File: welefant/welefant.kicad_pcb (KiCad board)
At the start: 2 copper layers, 80 x 90 mm, 72 parts, among them J1 Conn_02x11_Odd_Even, J2 Conn_02x11_Odd_Even, Q1 AO3400A, Q2 AO3401A, Q3 AO3401A, Q4 AO3400A, SW1 TS-1187A-B-A-B, SW2 TS-1187A-B-A-B, U1 ESP32-S3-WROOM-1-N8, U2 welefant, U3 XB8089D, U4 TP4056, U5 HE9073A33M5R, U6 MT3608L, U7 SK6812MINI-E_C5149201, U8 SK6812MINI-E_C5149201

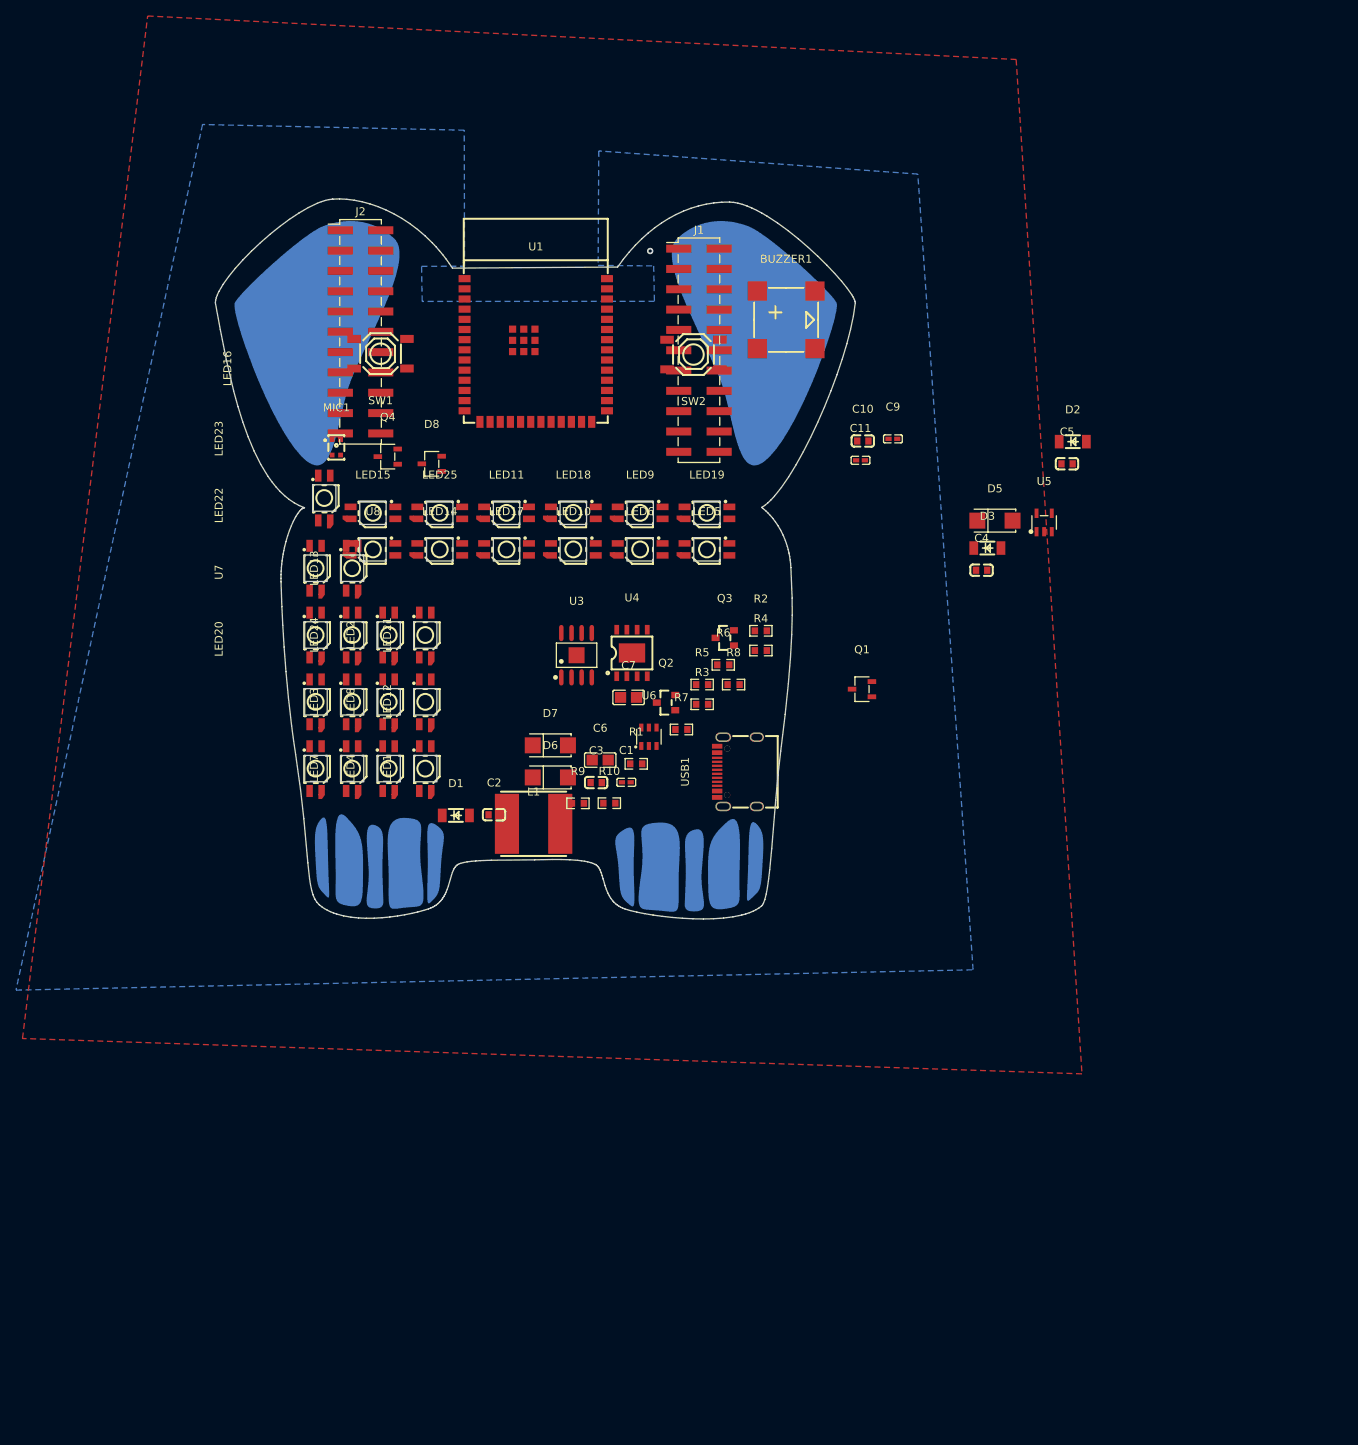
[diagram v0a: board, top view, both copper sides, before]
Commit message: blubb
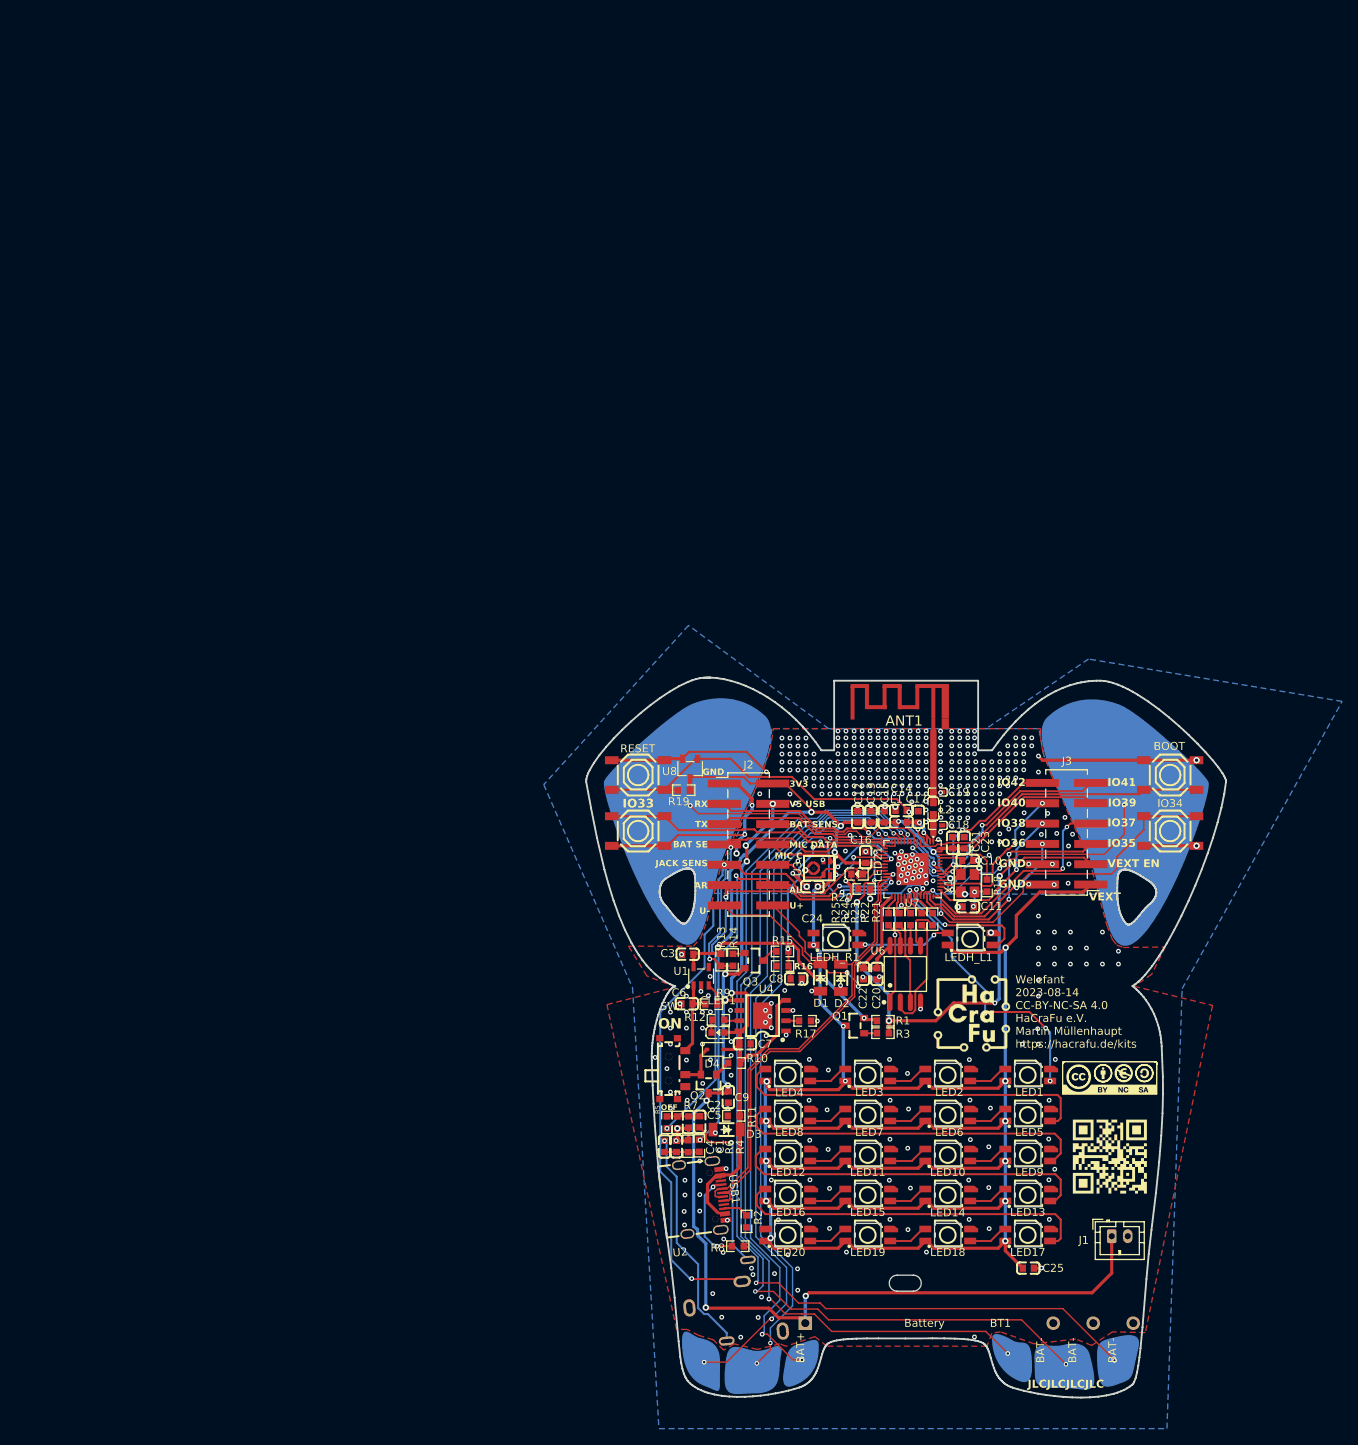
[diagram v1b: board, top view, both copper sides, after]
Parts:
- removed BUZZER1: MLT-8530, easyeda2kicad:BUZ-SMD_4P-L8.5-W8.5-P8.50-TL
- removed D5, D6, D7: SS34, easyeda2kicad:SMA_L4.3-W2.6-LS5.2-RD
- removed D8: BAV99,215, easyeda2kicad:SOT-23-3_L2.9-W1.6-P1.90-LS2.8-BR
- removed LED22, LED23, LED24, LED25: SK6812MINI-E, hacrafu:SK6812MINI-E-handsolder
- removed MIC1: ZTS6117, easyeda2kicad:MIC-SMD_4P-L2.8-W1.9-P1.84-TL_ZTS6117
- removed Q4: AO3400A, easyeda2kicad:SOT-23-3_L2.9-W1.6-P1.90-LS2.8-BR
- added ANT1: ANTENNA, hacrafu:antenna, F.Cu at (71.3, 36.8)
- added BT1: Battery, hacrafu:LiPo_Recycled_welefant, F.Cu at (59.4, 114.0)
- added C12: 10u, easyeda2kicad:C0603, F.Cu at (66.0, 50.7)
- added C13: 1u, easyeda2kicad:C0603, F.Cu at (67.6, 50.7)
- added C14: 1u, easyeda2kicad:C0603, F.Cu at (71.4, 49.9)
- added C15: 100n, easyeda2kicad:C0603, F.Cu at (69.3, 50.7)
- added C16: 100n, easyeda2kicad:C0603, F.Cu at (67.0, 55.8)
- added C17: 100n, easyeda2kicad:C0603, F.Cu at (73.5, 50.7)
- added C18: 4p7, easyeda2kicad:C0402, F.Cu at (76.0, 51.8)
- added C19: 3p3, easyeda2kicad:C0402, F.Cu at (76.0, 47.6)
- added C20: 100n, easyeda2kicad:C0603, F.Cu at (68.3, 70.3)
- added C21: 100n, easyeda2kicad:C0603, F.Cu at (77.8, 54.0)
- added C22: 1u, easyeda2kicad:C0603, F.Cu at (66.7, 70.3)
- added C23: 100n, easyeda2kicad:C0603, F.Cu at (79.2, 54.0)
- added C24: 100n, easyeda2kicad:C0603, F.Cu at (60.3, 59.5)
- added C25: 1u, easyeda2kicad:C0603, F.Cu at (87.3, 107.1)
- added C8: 10u, easyeda2kicad:C0603, F.Cu at (58.2, 71.0)
- added CLED1: yellow, easyeda2kicad:LED0603-RD-YELLOW, F.Cu at (48.5, 77.7)
- added D4: 1N5819WS, Diode_SMD:D_SOD-323, F.Cu at (48.1, 79.8)
- added J3: Conn_02x6_Odd_Even, hacrafu:PinHeader_2x06_P2.54mm_Vertical_SMD_handsolder, F.Cu at (92.0, 50.3)
- added L2: 2n2, easyeda2kicad:L0603, F.Cu at (75.4, 49.7)
- added LEDH_L1: SK6812MINI-E, hacrafu:SK6812MINI-E-handsolder, F.Cu at (80.0, 66.0)
- added LEDH_R1: SK6812MINI-E, hacrafu:SK6812MINI-E-handsolder, F.Cu at (63.2, 66.0)
- added R11: 10K, easyeda2kicad:R0603, F.Cu at (50.5, 88.1)
- added R12: 330, easyeda2kicad:R0603, F.Cu at (48.5, 76.1)
- added R13: 10K, easyeda2kicad:R0603, F.Cu at (48.9, 68.6)
- added R14: 1K, easyeda2kicad:R0603, F.Cu at (50.4, 68.6)
- added R15: 390K, easyeda2kicad:R0603, F.Cu at (56.5, 67.5)
- added R16: 100K, easyeda2kicad:R0603, F.Cu at (56.5, 69.4)
- added R17: 3K3, easyeda2kicad:R0603_NEW, F.Cu at (59.4, 76.2)
- added R18: 0, easyeda2kicad:R0603, F.Cu at (82.1, 59.3)
- added R19: 10K, easyeda2kicad:R0603, F.Cu at (44.2, 47.4)
- added R20: 330, easyeda2kicad:R0603, F.Cu at (66.8, 59.8)
- added R21: 0, easyeda2kicad:R0603, F.Cu at (75.3, 63.5)
- added R22: 0, easyeda2kicad:R0603, F.Cu at (74.0, 63.5)
- added R23: 0, easyeda2kicad:R0603, F.Cu at (72.5, 63.5)
- added R24: 0, easyeda2kicad:R0603, F.Cu at (71.2, 63.5)
- added R25: 0, easyeda2kicad:R0603, F.Cu at (69.8, 63.5)
- added SW3: BOOT, easyeda2kicad:SW-SMD_4P-L5.1-W5.1-P3.70-LS6.5-TL-2, F.Cu at (105.0, 45.5)
- added SW4: GPIO33, easyeda2kicad:SW-SMD_4P-L5.1-W5.1-P3.70-LS6.5-TL-2, F.Cu at (38.5, 52.5)
- added SW5: IO34, easyeda2kicad:SW-SMD_4P-L5.1-W5.1-P3.70-LS6.5-TL-2, F.Cu at (105.0, 52.5)
- added X1: 40 MHz, easyeda2kicad:OSC-SMD_4P-L3.2-W2.5-BL_SIT8008BI, F.Cu at (79.7, 59.0)
- C1: value 0.1u -> 33n; footprint easyeda2kicad:C0402_NEW -> easyeda2kicad:C0603
- C10: value 10u -> 15p
- C11: value 0.1u -> 15p; footprint easyeda2kicad:C0402_NEW -> easyeda2kicad:C0603
- C2: value 10u -> 33n
- C6: value 22u -> 1u; footprint easyeda2kicad:C0805 -> easyeda2kicad:C0603
- C7: value 22u -> 10u; footprint easyeda2kicad:C0805 -> easyeda2kicad:C0603
- C9: value 0.1u -> 10u; footprint easyeda2kicad:C0402_NEW -> easyeda2kicad:C0603
- D1: value 5V6 -> 3V3
- D3: value 3V3 -> 5V6
- J1: value Conn_02x11_Odd_Even -> Conn_01x02; footprint Connector_PinHeader_2.54mm:PinHeader_2x11_P2.54mm_Vertical_SMD -> Connector_JST:JST_PH_B2B-PH-K_1x02_P2.00mm_Vertical
- J2: value Conn_02x11_Odd_Even -> Conn_02x7_Odd_Even; footprint Connector_PinHeader_2.54mm:PinHeader_2x11_P2.54mm_Vertical_SMD -> hacrafu:PinHeader_2x07_P2.54mm_Vertical_SMD_handsolder
- L1: value 10u -> 2n2; footprint easyeda2kicad:IND-SMD_L8.0-W8.0 -> easyeda2kicad:L0603
- LED21: value SK6812MINI-E -> blue; footprint hacrafu:SK6812MINI-E-handsolder -> easyeda2kicad:LED0603-FD_BLUE
- Q1: value AO3400A -> AO3401A; footprint easyeda2kicad:SOT-23-3_L2.9-W1.6-P1.90-LS2.8-BR -> easyeda2kicad:SOT-23_L2.9-W1.3-P1.90-LS2.4-BR
- R1: value 5.1K -> 10K
- R10: value 10K -> 1K
- R2: value 1K -> 5.1K
- R3: value 5.1K -> 1K
- R4, R5: value 2.4K -> 270
- R6: value 10K -> 150
- R7: value 110K -> 150
- R8: value 110K -> 5.1K
- R9: value 15K -> 100K
- SW1: value TS-1187A-B-A-B -> ON-OFF; footprint easyeda2kicad:SW-SMD_4P-L5.1-W5.1-P3.70-LS6.5-TL-2 -> easyeda2kicad:SW-TH_K3-1296S-E1
- SW2: value TS-1187A-B-A-B -> RESET
- U1: value ESP32-S3-WROOM-1-N8 -> RT9080-33GJ5; footprint easyeda2kicad:WIFIM-SMD_ESP32-S3-WROOM-1-N8 -> easyeda2kicad:TSOT-23-5_L2.9-W1.6-P0.95-LS2.8-BL
- U2: value welefant -> Audio Jack PJ-324; footprint hacrafu:welefant -> easyeda2kicad:AUDIO-TH_PJ-32400
- U3: value XB8089D -> SD18OB261-060; footprint easyeda2kicad:SOIC-8_L5.0-W4.0-P1.27-LS6.0-BL-EP2.0 -> hacrafu:MIC-SMD_SD18OB261-060
- U5: value HE9073A33M5R -> welefant; footprint easyeda2kicad:SOT-23-5_L3.0-W1.7-P0.95-LS2.8-BL -> hacrafu:welefant; moved to B.Cu
- U6: value MT3608L -> 128MBit Flash; footprint easyeda2kicad:SOT-23-6_L2.9-W1.7-P0.95-LS2.8-BL -> easyeda2kicad:SOIC-8_L5.3-W5.3-P1.27-LS8.0-BL
- U7: value SK6812MINI-E_C5149201 -> ESP32-S3; footprint hacrafu:SK6812MINI-E-handsolder -> easyeda2kicad:QFN-56_L7.0-W7.0-P0.40-TL-EP4.0
- U8: value SK6812MINI-E_C5149201 -> Reset 2.8V; footprint hacrafu:SK6812MINI-E-handsolder -> easyeda2kicad:SOT-23-3_L2.9-W1.6-P1.90-LS2.8-BR
- moved J1 122.2 mm to (97.7, 103.2)
- moved LED13 115.2 mm to (87.2, 98.0), turned to 180 degrees
- moved LED17 107.7 mm to (87.2, 103.0), turned to 180 degrees
- moved LED15 105.3 mm to (67.2, 98.0), turned to 180 degrees
- moved LED16 104.6 mm to (57.2, 98.0), turned to 180 degrees
- moved LED14 102.7 mm to (77.2, 98.0), turned to 180 degrees
- moved LED18 101.7 mm to (77.2, 103.0), turned to 180 degrees
- moved SW1 96.5 mm to (42.8, 82.2), turned to 0 degrees
- moved U2 96.0 mm to (50.5, 111.2), turned to 6 degrees
- moved C5 94.2 mm to (46.2, 88.8), turned to -90 degrees
- moved LED9 93.8 mm to (87.2, 93.0), turned to 180 degrees
- moved LED19 92.5 mm to (67.2, 103.0), turned to 180 degrees
- moved LED11 92.1 mm to (67.2, 93.0), turned to 180 degrees
- moved LED10 89.0 mm to (77.2, 93.0), turned to 180 degrees
- moved LED2 88.9 mm to (77.2, 83.0), turned to 180 degrees
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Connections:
- C1 pad 1: Net-(C1-Pad1) -> GND
- C10 pad 1: Net-(BUZZER1-Pad1) -> /XTAL_N
- C10 pad 2: /GND -> GND
- C11 pad 1: Net-(R14-Pad2) -> GND
- C2 pad 1: /Power/VBAT -> GND
- C2 pad 2: /GND -> Net-(C2-Pad2)
- C3 pad 1: /Power/VUSB -> GND
- C3 pad 2: /GND -> /V33
- C4 pad 1: Net-(Q2-Pad2) -> Net-(C1-Pad2)
- C4 pad 2: /GND -> Net-(C4-Pad2)
- C5 pad 1: /GND -> Net-(C2-Pad2)
- C5 pad 2: /Power/V33 -> Net-(C5-Pad2)
- C6 pad 1: /Power/V5 -> GND
- C6 pad 2: /GND -> /VBUS
- C7 pad 1: Net-(C7-Pad1) -> /V5
- C7 pad 2: /GND -> GND
- C9 pad 1: /VEXT -> GND
- C9 pad 2: /GND -> /VBAT
- D1 pad 1: /Power/VUSB -> /USB_DP
- D1 pad 2: /GND -> GND
- D2 pad 1: /Power/USB_DP -> /USB_DN
- D2 pad 2: /GND -> GND
- D3 pad 1: /Power/USB_DN -> /V5
- D3 pad 2: /GND -> GND
- J1 pad 1: unconnected-(J1-Pad1) -> /VBAT
- J1 pad 2: unconnected-(J1-Pad2) -> GND
- J2 pad 1: unconnected-(J2-Pad1) -> GND
- J2 pad 10: unconnected-(J2-Pad10) -> /MIC_CLK
- J2 pad 11: unconnected-(J2-Pad11) -> /AUDIO_PWM_R
- J2 pad 12: unconnected-(J2-Pad12) -> /AUDIO_PWM_L
- J2 pad 13: unconnected-(J2-Pad13) -> /USB_DP
- J2 pad 14: unconnected-(J2-Pad14) -> /USB_DN
- J2 pad 2: unconnected-(J2-Pad2) -> /V33
- J2 pad 3: unconnected-(J2-Pad3) -> /RX
- J2 pad 4: unconnected-(J2-Pad4) -> /V5
- J2 pad 5: unconnected-(J2-Pad5) -> /TX
- J2 pad 6: unconnected-(J2-Pad6) -> /BAT_SENS
- J2 pad 7: unconnected-(J2-Pad7) -> /BAT_SENS_EN
- J2 pad 8: unconnected-(J2-Pad8) -> /MIC_DATA
- J2 pad 9: unconnected-(J2-Pad9) -> /JACK_SENS
- L1 pad 1: Net-(D7-Pad2) -> /V33
- L1 pad 2: Net-(C7-Pad1) -> Net-(C17-Pad2)
- LED1 pad 1: /LEDs/VUSB -> /VEXT
- LED1 pad 2: unconnected-(LED1-Pad2) -> Net-(LED1-DOUT)
- LED1 pad 3: /LEDs/GND -> GND
- LED1 pad 4: Net-(LED1-Pad4) -> /LED_MATRIX
- LED10 pad 1: /LEDs/VUSB -> /VEXT
- LED10 pad 2: Net-(LED10-Pad2) -> Net-(LED10-DOUT)
- LED10 pad 3: /LEDs/GND -> GND
- LED10 pad 4: unconnected-(LED10-Pad4) -> Net-(LED10-DIN)
- LED11 pad 1: /LEDs/VUSB -> /VEXT
- LED11 pad 2: unconnected-(LED11-Pad2) -> Net-(LED11-DOUT)
- LED11 pad 3: /LEDs/GND -> GND
- LED11 pad 4: Net-(LED11-Pad4) -> Net-(LED10-DOUT)
- LED12 pad 1: /LEDs/VUSB -> /VEXT
- LED12 pad 2: Net-(LED11-Pad4) -> /D3_LED
- LED12 pad 3: /LEDs/GND -> GND
- LED12 pad 4: Net-(LED12-Pad4) -> Net-(LED11-DOUT)
- LED13 pad 1: /LEDs/VUSB -> /VEXT
- LED13 pad 2: Net-(LED12-Pad4) -> Net-(LED13-DOUT)
- LED13 pad 3: /LEDs/GND -> GND
- LED13 pad 4: Net-(LED13-Pad4) -> /D3_LED
- LED14 pad 1: /LEDs/VUSB -> /VEXT
- LED14 pad 2: Net-(LED13-Pad4) -> Net-(LED14-DOUT)
- LED14 pad 3: /LEDs/GND -> GND
- LED14 pad 4: Net-(LED14-Pad4) -> Net-(LED13-DOUT)
- LED15 pad 1: /LEDs/VUSB -> /VEXT
- LED15 pad 2: Net-(LED14-Pad4) -> Net-(LED15-DOUT)
- LED15 pad 3: /LEDs/GND -> GND
- LED15 pad 4: unconnected-(LED15-Pad4) -> Net-(LED14-DOUT)
- LED16 pad 1: /LEDs/VUSB -> /VEXT
- LED16 pad 2: unconnected-(LED16-Pad2) -> /D4_LED
- LED16 pad 3: /LEDs/GND -> GND
- LED16 pad 4: Net-(LED16-Pad4) -> Net-(LED15-DOUT)
- LED17 pad 1: /LEDs/VUSB -> /VEXT
- LED17 pad 2: Net-(LED16-Pad4) -> Net-(LED17-DOUT)
- LED17 pad 3: /LEDs/GND -> GND
- LED17 pad 4: Net-(LED17-Pad4) -> /D4_LED
- LED18 pad 1: /LEDs/VUSB -> /VEXT
- LED18 pad 2: Net-(LED17-Pad4) -> Net-(LED18-DOUT)
- LED18 pad 3: /LEDs/GND -> GND
- LED18 pad 4: Net-(LED18-Pad4) -> Net-(LED17-DOUT)
- LED19 pad 1: /LEDs/VUSB -> /VEXT
- LED19 pad 2: Net-(LED18-Pad4) -> Net-(LED19-DOUT)
- LED19 pad 3: /LEDs/GND -> GND
- LED19 pad 4: Net-(LED19-Pad4) -> Net-(LED18-DOUT)
- LED2 pad 1: /LEDs/VUSB -> /VEXT
- LED2 pad 2: Net-(LED1-Pad4) -> Net-(LED2-DOUT)
- LED2 pad 3: /LEDs/GND -> GND
- LED2 pad 4: Net-(LED2-Pad4) -> Net-(LED1-DOUT)
- LED20 pad 1: /LEDs/VUSB -> /VEXT
- LED20 pad 2: Net-(LED19-Pad4) -> unconnected-(LED20-DOUT-Pad2)
- LED20 pad 3: /LEDs/GND -> GND
- LED20 pad 4: unconnected-(LED20-Pad4) -> Net-(LED19-DOUT)
- LED21 pad 1: /LEDs/VUSB -> Net-(LED21-C)
- LED21 pad 2: unconnected-(LED21-Pad2) -> /LED
- LED3 pad 1: /LEDs/VUSB -> /VEXT
- LED3 pad 2: Net-(LED2-Pad4) -> Net-(LED3-DOUT)
- LED3 pad 3: /LEDs/GND -> GND
- LED3 pad 4: Net-(LED3-Pad4) -> Net-(LED2-DOUT)
- LED4 pad 1: /LEDs/VUSB -> /VEXT
- LED4 pad 2: Net-(LED3-Pad4) -> /D1_LED
- LED4 pad 3: /LEDs/GND -> GND
- LED4 pad 4: Net-(LED4-Pad4) -> Net-(LED3-DOUT)
- LED5 pad 1: /LEDs/VUSB -> /VEXT
- LED5 pad 2: Net-(LED4-Pad4) -> Net-(LED5-DOUT)
- LED5 pad 3: /LEDs/GND -> GND
- LED5 pad 4: unconnected-(LED5-Pad4) -> /D1_LED
- LED6 pad 1: /LEDs/VUSB -> /VEXT
- LED6 pad 2: unconnected-(LED6-Pad2) -> Net-(LED6-DOUT)
- LED6 pad 3: /LEDs/GND -> GND
- LED6 pad 4: Net-(LED6-Pad4) -> Net-(LED5-DOUT)
- LED7 pad 1: /LEDs/VUSB -> /VEXT
- LED7 pad 2: Net-(LED6-Pad4) -> Net-(LED7-DOUT)
- LED7 pad 3: /LEDs/GND -> GND
- LED7 pad 4: Net-(LED7-Pad4) -> Net-(LED6-DOUT)
- LED8 pad 1: /LEDs/VUSB -> /VEXT
- LED8 pad 2: Net-(LED7-Pad4) -> /D2_LED
- LED8 pad 3: /LEDs/GND -> GND
- LED8 pad 4: Net-(LED8-Pad4) -> Net-(LED7-DOUT)
- LED9 pad 1: /LEDs/VUSB -> /VEXT
- LED9 pad 2: Net-(LED8-Pad4) -> Net-(LED10-DIN)
- LED9 pad 3: /LEDs/GND -> GND
- LED9 pad 4: Net-(LED10-Pad2) -> /D2_LED
- Q1 pad 1: /VEXT_EN -> Net-(Q1-G)
- Q1 pad 2: /Power/V33 -> /V33
- Q2 pad 1: /Power/VUSB -> Net-(Q2-G)
- Q2 pad 2: Net-(Q2-Pad2) -> Net-(D4-K)
- Q2 pad 3: /Power/VBAT -> /VBAT
- Q3 pad 1: /Power/VUSB -> Net-(Q3-G)
- Q3 pad 2: Net-(C7-Pad1) -> /VBAT
- Q3 pad 3: /Power/VBAT -> Net-(Q3-D)
- R1 pad 1: /GND -> /V33
- R1 pad 2: Net-(R1-Pad2) -> /VEXT_EN
- R10 pad 1: /GND -> Net-(Q2-G)
- R10 pad 2: /Power/VUSB -> /V5
- R2 pad 1: /Power/VBAT -> GND
- R2 pad 2: Net-(C1-Pad2) -> Net-(USB1-CC2)
- R3 pad 1: Net-(R3-Pad1) -> Net-(Q1-G)
- R3 pad 2: /GND -> /VEXT_EN
- R4 pad 1: Net-(D4-Pad1) -> /AUDIO_PWM_L
- R4 pad 2: Net-(R4-Pad2) -> Net-(C1-Pad2)
- R5 pad 1: Net-(R5-Pad1) -> /AUDIO_PWM_R
- R5 pad 2: /GND -> Net-(C2-Pad2)
- R6 pad 1: /Power/VUSB -> GND
- R6 pad 2: /GND -> Net-(C1-Pad2)
- R7 pad 1: Net-(R7-Pad1) -> GND
- R7 pad 2: /Power/V5 -> Net-(C2-Pad2)
- R8 pad 1: Net-(R8-Pad1) -> Net-(USB1-CC1)
- R8 pad 2: /GND -> GND
- R9 pad 1: /GND -> Net-(U1-EN)
- R9 pad 2: Net-(R7-Pad1) -> /VBUS
- SW1 pad 1: /EN -> unconnected-(SW1-Pad1)
- SW1 pad 2: unconnected-(SW1-Pad2) -> Net-(D4-K)
- SW1 pad 3: /GND -> /VBUS
- SW2 pad 1: /IO0 -> /RESET
- SW2 pad 2: unconnected-(SW2-Pad2) -> /RESET
- SW2 pad 3: /GND -> GND
- SW2 pad 4: unconnected-(SW2-Pad4) -> GND
- U1 pad 1: /GND -> /VBUS
- U1 pad 2: /Power/V33 -> GND
- U1 pad 3: /EN -> Net-(U1-EN)
- U1 pad 5: unconnected-(U1-Pad5) -> /V33
- U2 pad 1: unconnected-(U2-Pad1) -> GND
- U2 pad 2: unconnected-(U2-Pad2) -> Net-(C5-Pad2)
- U2 pad 3: unconnected-(U2-Pad3) -> /JACK_SENS
- U2 pad 5: unconnected-(U2-Pad5) -> Net-(C4-Pad2)
- U3 pad 1: /GND -> /MIC_DATA
- U3 pad 2: /GND -> GND
- U3 pad 3: /GND -> GND
- U3 pad 4: /GND -> /MIC_CLK
- U3 pad 5: Net-(C1-Pad1) -> /VEXT
- U4 pad 1: /GND -> GND
- U4 pad 2: Net-(R5-Pad1) -> Net-(U4-PROG)
- U4 pad 3: /GND -> GND
- U4 pad 4: /Power/VUSB -> /V5
- U4 pad 5: /Power/VBAT -> /VBAT
- U4 pad 7: Net-(R4-Pad2) -> Net-(U4-~{CHRG})
- U4 pad 8: /Power/VUSB -> /V5
- U4 pad 9: unconnected-(U4-Pad9) -> GND
- U5 pad 1: Net-(Q2-Pad2) -> /TOUCH_EL
- U5 pad 2: /GND -> /TOUCH_ER
- U5 pad 3: Net-(Q2-Pad2) -> /TOUCH_T1
- U5 pad 4: unconnected-(U5-Pad4) -> /TOUCH_T2
- U5 pad 5: /Power/V33 -> /TOUCH_T3
- U6 pad 1: Net-(D7-Pad2) -> /SPICS0
- U6 pad 2: /GND -> /SPIQ
- U6 pad 3: Net-(R7-Pad1) -> /SPIWP
- U6 pad 4: /Power/V5_EN -> GND
- U6 pad 5: Net-(C7-Pad1) -> /SPID
- U6 pad 6: Net-(R8-Pad1) -> /SPICLK
- U7 pad 1: /LEDs/VUSB -> Net-(U7-LNA_IN)
- U7 pad 2: unconnected-(U7-Pad2) -> Net-(C17-Pad2)
- U7 pad 3: /LEDs/GND -> Net-(C17-Pad2)
- U7 pad 4: Net-(U7-Pad4) -> /RESET
- U8 pad 1: /LEDs/VUSB -> /RESET
- U8 pad 2: Net-(U7-Pad4) -> GND
- U8 pad 3: /LEDs/GND -> /V33
- USB1 pad 1: (no net) -> unconnected-(USB1-SH-Pad1)
- USB1 pad A1: /GND -> GND
- USB1 pad A12: /GND -> GND
- USB1 pad A4: /Power/VUSB -> /V5
- USB1 pad A5: Net-(R3-Pad1) -> Net-(USB1-CC1)
- USB1 pad A6: /Power/USB_DP -> /USB_DP
- USB1 pad A7: /Power/USB_DN -> /USB_DN
- USB1 pad A9: /Power/VUSB -> /V5
- USB1 pad B1: /GND -> GND
- USB1 pad B12: /GND -> GND
- USB1 pad B4: /Power/VUSB -> /V5
- USB1 pad B5: Net-(R1-Pad2) -> Net-(USB1-CC2)
- USB1 pad B6: /Power/USB_DP -> /USB_DP
- USB1 pad B7: /Power/USB_DN -> /USB_DN
- USB1 pad B9: /Power/VUSB -> /V5
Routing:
- net /VEXT: track 0.00 -> 275.1 mm, vias 0 -> 15
- net /TOUCH_T1: track 0.00 -> 127.9 mm, vias 0 -> 3
- net /TOUCH_T2: track 0.00 -> 121.3 mm, vias 0 -> 3
- net /V33: track 0.00 -> 113.3 mm, vias 0 -> 9
- net /VBAT: track 0.00 -> 110.6 mm, vias 0 -> 6
- net /TOUCH_T3: track 0.00 -> 110.3 mm, vias 0 -> 3
- net GND: track 0.00 -> 101.2 mm, vias 0 -> 458
- net /JACK_SENS: track 0.00 -> 89.6 mm, vias 0 -> 2
- net /TOUCH_T6: track 0.00 -> 88.5 mm, vias 0 -> 3
- net /TOUCH_T4: track 0.00 -> 88.2 mm, vias 0 -> 3
- net /TOUCH_T5: track 0.00 -> 83.2 mm, vias 0 -> 3
- net /V5: track 0.00 -> 76.0 mm, vias 0 -> 4
- net /USB_DP: track 0.00 -> 74.6 mm, vias 0 -> 2
- net /VEXT_EN: track 0.00 -> 70.0 mm, vias 0 -> 6
- net /USB_DN: track 0.00 -> 66.4 mm
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- added copper zone on B.Cu, net GND
- added copper zone on F.Cu, net GND
- removed copper zone on B.Cu, net /GND
- removed copper zone on F.Cu, net /GND
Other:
- outline, holes or cut-outs redrawn
- board text added: "3V3"
- board text added: "AL"
- board text added: "AR"
- board text added: "BAT SE"
- board text added: "BAT SENS"
- board text added: "GND"
- board text added: "IO33"
- board text added: "IO34"
- board text added: "IO35"
- board text added: "IO36"
- board text added: "IO37"
- board text added: "IO38"
- board text added: "IO39"
- board text added: "IO40"
- board text added: "IO41"
- board text added: "IO42"
- board text added: "JACK SENS"
- board text added: "JLCJLCJLCJLC"
- board text added: "MIC C"
- board text added: "MIC DATA"
- board text added: "OFF"
- board text added: "ON"
- board text added: "RX"
- board text added: "TX"
- board text added: "U+"
- board text added: "U-"
- board text added: "V5 USB"
- board text added: "VEXT"
- board text added: "VEXT EN"
- board text added: "Welefant ${ISSUE_DATE} CC-BY-NC-SA 4.0 HaCraFu e.V. Martin Müllenhaupt https://hacrafu.de/kits"
